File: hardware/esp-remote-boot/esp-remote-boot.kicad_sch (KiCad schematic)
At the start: 10 parts, among them J1 Header IN, J2 Power Connector, J3 Header OUT, J5 USB C 2.0, U1 Button Trigger, U2 LED Sensor

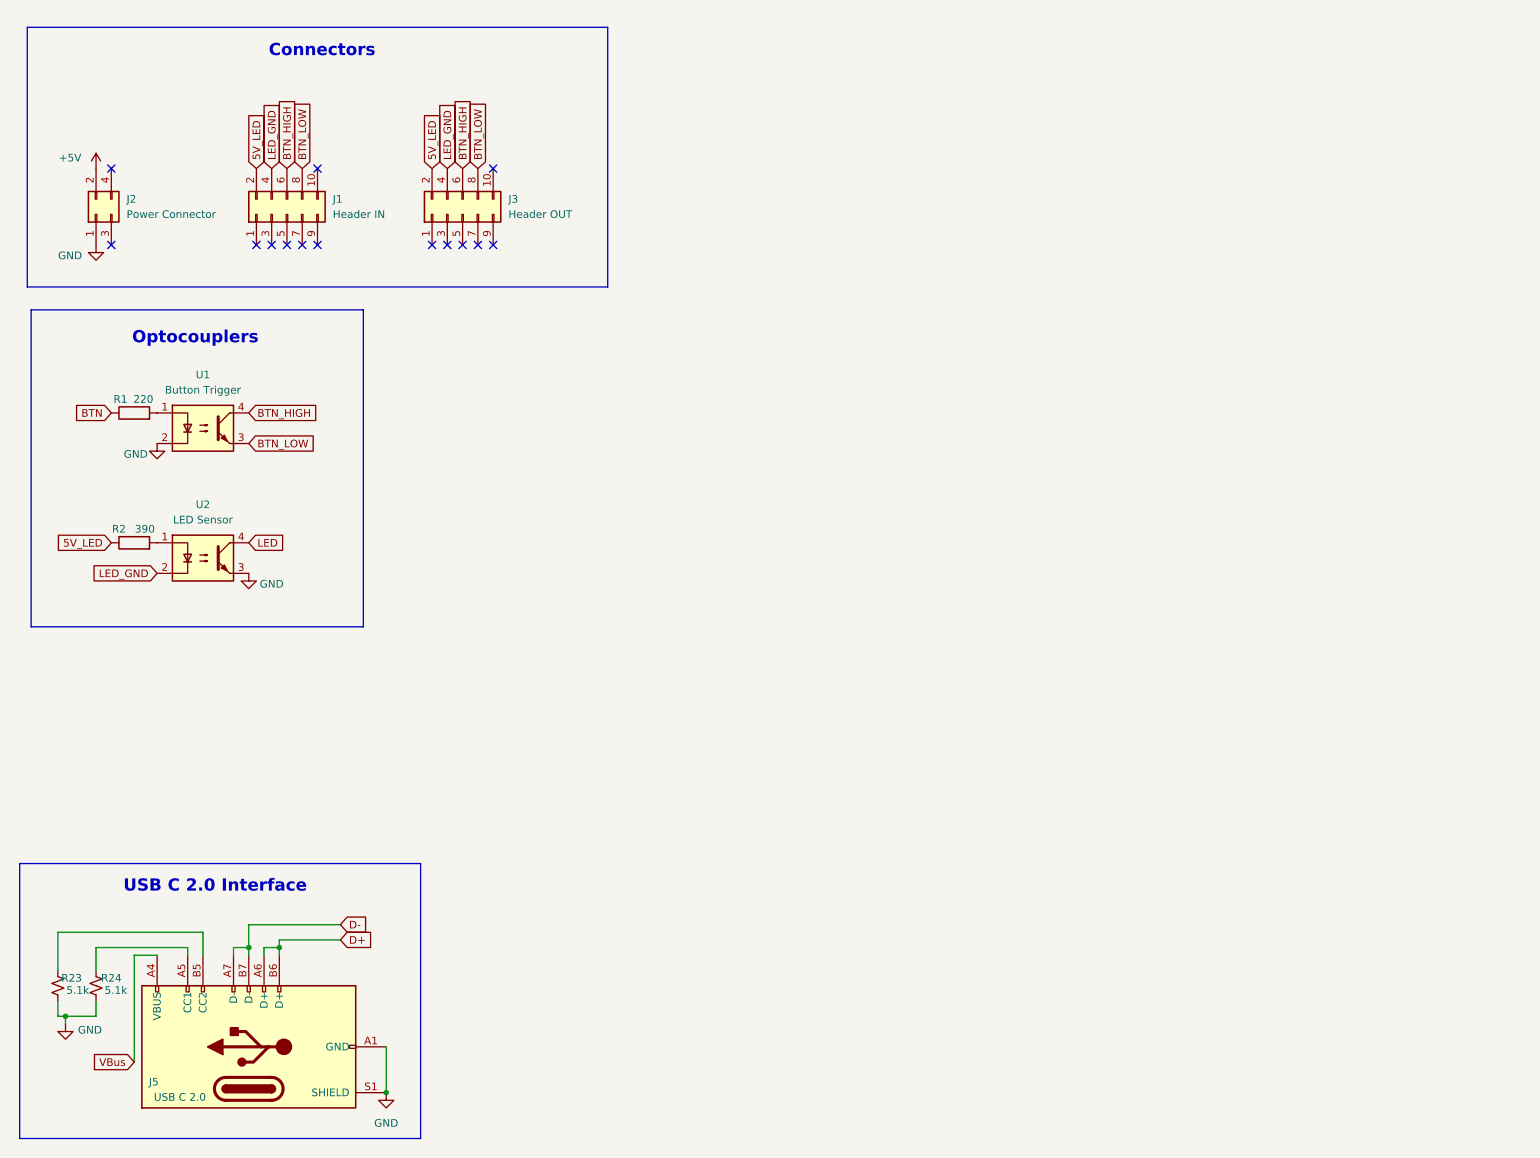
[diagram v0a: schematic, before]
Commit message: Minor USB C Changes
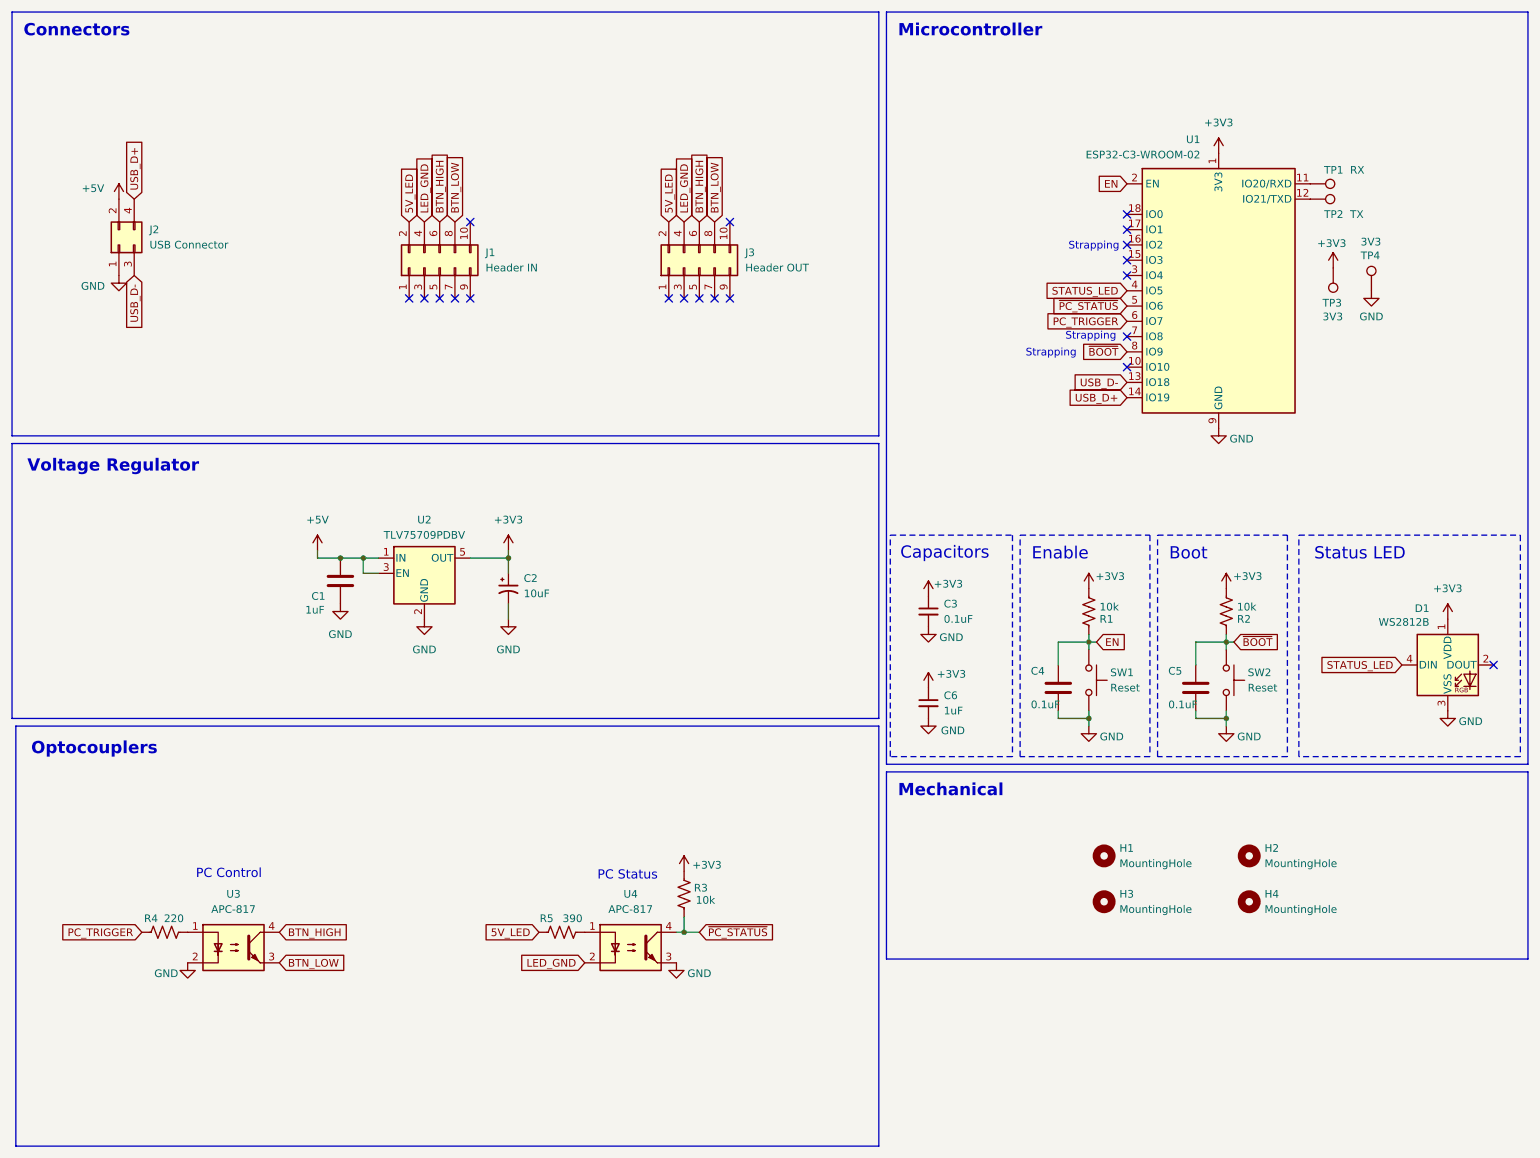
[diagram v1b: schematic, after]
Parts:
- removed J5: USB C 2.0, Connector_USB:USB_C_Receptacle_G-Switch_GT-USB-7010ASV, symbol Connector:USB_C_Receptacle_USB2.0_14P
- removed R23, R24: 5.1k, Resistor_SMD:R_0805_2012Metric_Pad1.20x1.40mm_HandSolder, symbol Device:R_Small_US
- removed U1: Button Trigger, Package_DIP:DIP-4_W7.62mm, symbol Isolator:PC817
- removed U2: LED Sensor, Package_DIP:DIP-4_W7.62mm, symbol Isolator:PC817
- added C1: 1uF, Capacitor_SMD:C_0805_2012Metric_Pad1.18x1.45mm_HandSolder, symbol Device:C
- added C2: 10uF, Capacitor_SMD:C_0805_2012Metric_Pad1.18x1.45mm_HandSolder, symbol Device:C_Polarized_Small_US
- added C3: 0.1uF, Capacitor_SMD:C_0805_2012Metric_Pad1.18x1.45mm_HandSolder, symbol Device:C_Small
- added C4, C5: 0.1uF, Capacitor_SMD:C_0805_2012Metric_Pad1.18x1.45mm_HandSolder, symbol Device:C
- added C6: 1uF, Capacitor_SMD:C_0805_2012Metric_Pad1.18x1.45mm_HandSolder, symbol Device:C_Small
- added D1: WS2812B, LED_SMD:LED_WS2812B_PLCC4_5.0x5.0mm_P3.2mm, symbol LED:WS2812B
- added H1, H2, H3, H4: MountingHole, MountingHole:MountingHole_3.2mm_M3, symbol Mechanical:MountingHole
- added R1, R2, R3: 10k, Resistor_SMD:R_0805_2012Metric_Pad1.20x1.40mm_HandSolder, symbol Device:R_US
- added SW1, SW2: Reset, Button_Switch_SMD:SW_SPST_PTS810, symbol Switch:SW_Push
- added TP1: RX, TestPoint:TestPoint_Pad_1.5x1.5mm, symbol Connector:TestPoint
- added TP2: TX, TestPoint:TestPoint_Pad_1.5x1.5mm, symbol Connector:TestPoint
- added TP3, TP4: 3V3, TestPoint:TestPoint_Pad_1.5x1.5mm, symbol Connector:TestPoint
- added U1: ESP32-C3-WROOM-02, RF_Module:ESP32-C3-WROOM-02, symbol RF_Module:ESP32-C3-WROOM-02
- added U2: TLV75709PDBV, Package_TO_SOT_SMD:SOT-23-5, symbol Regulator_Linear:TLV75709PDBV
- added U3, U4: APC-817, Package_DIP:SMDIP-4_W9.53mm, symbol Isolator:Optocoupler_DC_PhotoNPN_AKEC
- J2: value Power Connector -> USB Connector
- R4: renamed from R1; footprint (none) -> Resistor_SMD:R_0805_2012Metric_Pad1.20x1.40mm_HandSolder; symbol Device:R -> Device:R_US
- R5: renamed from R2; footprint (none) -> Resistor_SMD:R_0805_2012Metric_Pad1.20x1.40mm_HandSolder; symbol Device:R -> Device:R_US
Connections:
- net +5V: now also C1.1, U2.1 (IN), U2.3 (EN)
- net BTN_HIGH: now also U3.4
- net BTN_LOW: now also U3.3
- net GND: now also C1.2, C2.2, C3.2, C4.2, C5.2, C6.2, D1.3 (VSS), SW1.2, SW2.2, TP4.1, U1.19 (GND), U1.9 (GND), U2.2 (GND), U3.2, U4.3
- net LED_GND: now also U4.2
- net at R5.2: now also U4.1
- net at R4.2: now also U3.1
- net USB_D-: now reaches J2.3 (Pin_3)
- net USB_D-: now also U1.13 (IO18)
- net USB_D+: now reaches J2.4 (Pin_4)
- net USB_D+: now also U1.14 (IO19)
- net BTN renamed PC_TRIGGER
- net PC_TRIGGER: now also U1.6 (IO7)
- new net: TP1.1, U1.11 (IO20/RXD)
- new net: TP2.1, U1.12 (IO21/TXD)
- new net +3V3: C2.1, C3.1, C6.1, D1.1 (VDD), R1.2, R2.2, R3.2, TP3.1, U1.1 (3V3), U2.5 (OUT)
- new net EN: C4.1, R1.1, SW1.1, U1.2 (EN)
- new net STATUS_LED: D1.4 (DIN), U1.4 (IO5)
- new net ~{BOOT}: C5.1, R2.1, SW2.1, U1.8 (IO9)
- new net ~{PC_STATUS}: R3.1, U1.5 (IO6), U4.4
- no-connect marks 14 -> 20
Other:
- note added: "Boot"
- note added: "Capacitors"
- note added: "Enable"
- note added: "Mechanical"
- note added: "Microcontroller"
- note added: "PC Control"
- note added: "PC Status"
- note added: "Status LED"
- note added: "Strapping"
- note added: "Voltage Regulator"
- note removed: "USB C 2.0 Interface"
- title: ESP8266 PC Remote Boot Board -> ESP32 PC Remote Boot Board
- moved on the sheet: J1, J2, J3
